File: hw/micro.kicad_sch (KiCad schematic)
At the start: 66 parts, among them J5 USB_C_Receptacle, J6 Conn_ST_STDC14, J7 TC2070, Q2 2N7002, SW2 MCU Reset, SW3 User1, SW4 SW_Nidec_CAS-120A1, U8 STSPIN32G4, U9 BNO055, Y1 25MHz

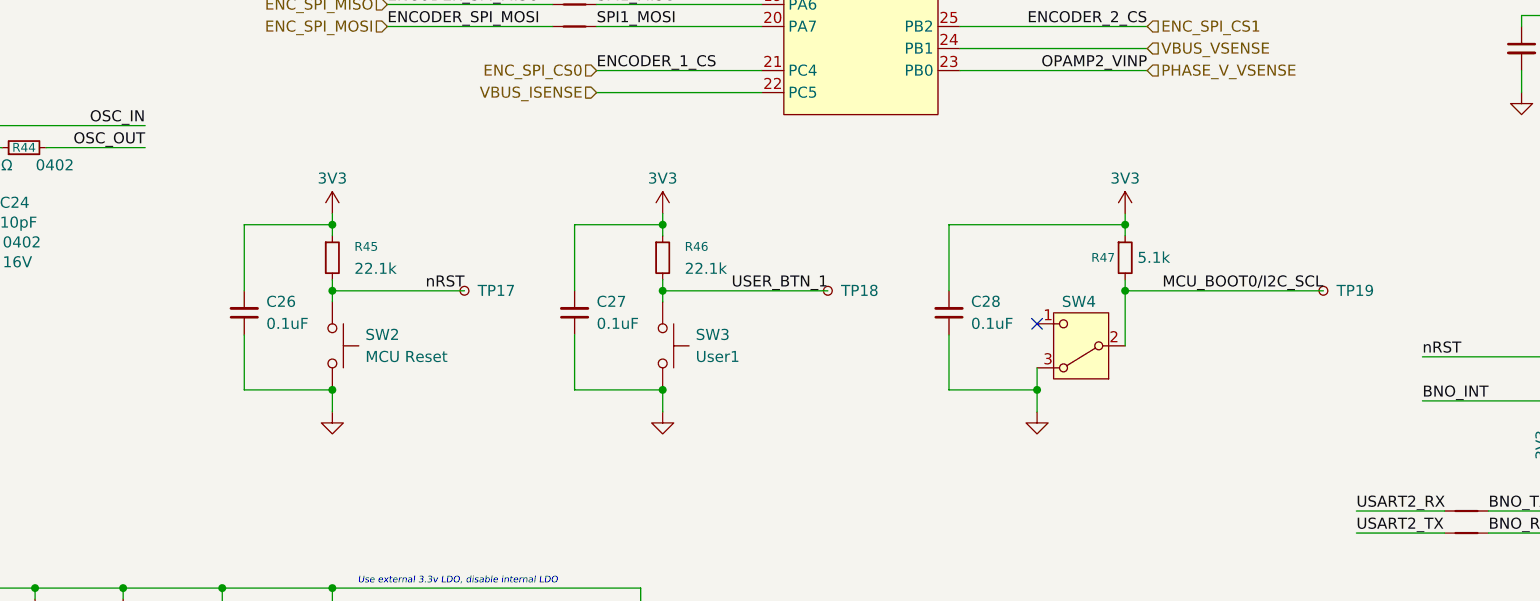
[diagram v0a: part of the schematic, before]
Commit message: More layout
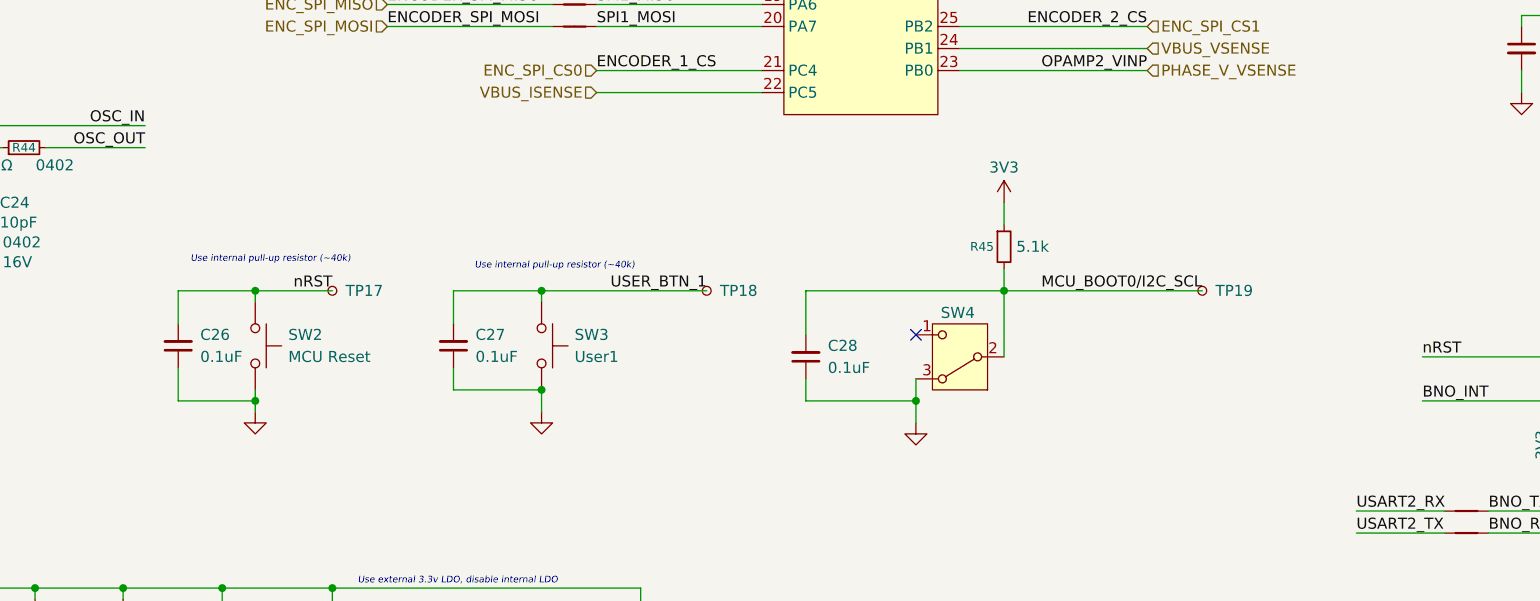
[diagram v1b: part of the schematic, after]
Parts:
- removed R45, R46: 22.1k, Resistor_SMD:R_0402_1005Metric, symbol Device:R_Small
- renumbered R47 to R45
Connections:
- net 3V3: no longer C26.2, C27.2, C28.2
- net I2C_SCL: now also C28.2
- net USER_BTN_1: now also C27.2
- net nRST: now also C26.2
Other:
- note added: "Use internal pull-up resistor (~40k)"
- moved on the sheet: C26, C27, C28, R45, SW2, SW3, SW4, TP17, TP18, TP19
